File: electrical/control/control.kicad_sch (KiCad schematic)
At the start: 45 parts, among them J1 USB4105-GF-A, J3 SWD, J4 QWIIC, J5 TC2030-NL, J6 UART, SW1 SYS, U1 RP2040, U2 ABPMRRV001PD2A3, U4 W25Q16JVSSIQ, U5 LP5907MFX-3.3, Y1 ABM8-272-T3

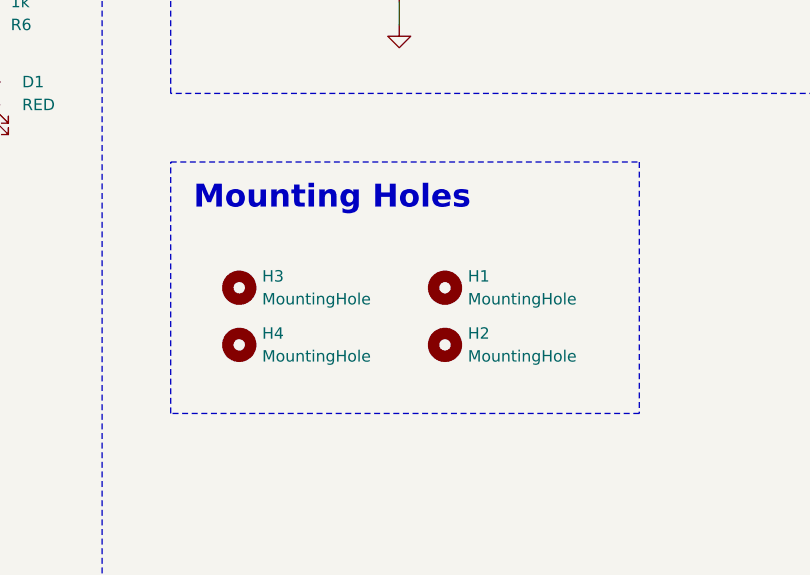
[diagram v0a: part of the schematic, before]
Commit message: Reduce number of mounting holes
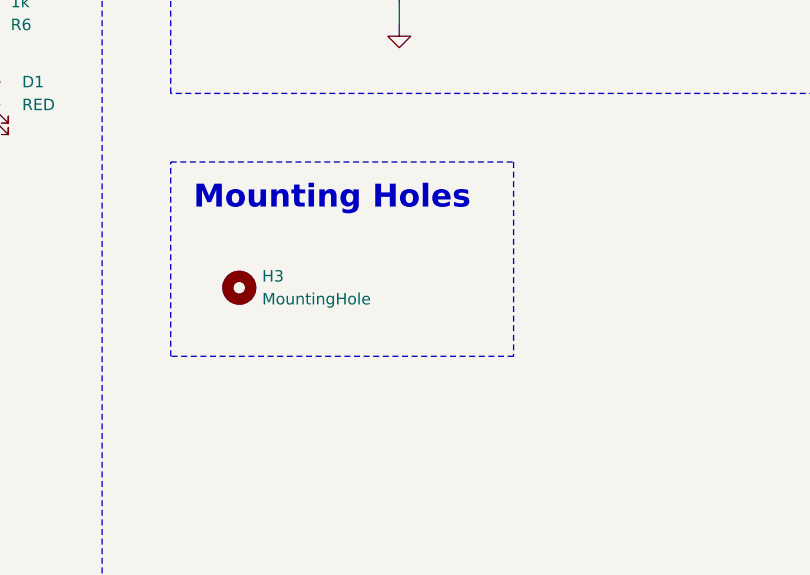
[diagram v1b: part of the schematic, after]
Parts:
- removed H1, H2, H4: MountingHole, MountingHole:MountingHole_3.2mm_M3, symbol Mechanical:MountingHole
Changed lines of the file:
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@@
 	(rectangle
 		(start 300.99 158.75)
-		(end 353.06 186.69)
+		(end 339.09 180.34)
 		(stroke
 			(width 0)
@@
 	)
 	(symbol
-		(lib_id "Mechanical:MountingHole")
-		(at 331.47 172.72 0)
-		(unit 1)
-		(exclude_from_sim no)
-		(in_bom no)
-		(on_board yes)
-		(dnp no)
-		(fields_autoplaced yes)
-		(property "Reference" "H1"
-			(at 334.01 171.4499 0)
-			(effects
-				(font
-					(size 1.27 1.27)
-				)
-				(justify left)
-			)
-		)
-		(property "Value" "MountingHole"
-			(at 334.01 173.9899 0)
-			(effects
-				(font
-					(size 1.27 1.27)
-				)
-				(justify left)
-			)
-		)
-		(property "Footprint" "MountingHole:MountingHole_3.2mm_M3"
-			(at 331.47 172.72 0)
-			(effects
-				(font
-					(size 1.27 1.27)
-				)
-				(hide yes)
-			)
-		)
-		(property "Datasheet" "~"
-			(at 331.47 172.72 0)
-			(effects
-				(font
-					(size 1.27 1.27)
-				)
-				(hide yes)
-			)
-		)
-		(property "Description" "Mounting Hole without connection"
-			(at 331.47 172.72 0)
-			(effects
-				(font
-					(size 1.27 1.27)
-				)
-				(hide yes)
-			)
-		)
-		(instances
-			(project "control"
-				(path "/da26d94e-7a50-4b99-9678-5aaaf6987a15"
-					(reference "H1")
-					(unit 1)
-				)
-			)
-		)
-	)
-	(symbol
 		(lib_id "Device:R_US")
 		(at 105.41 83.82 0)
@@
 	)
 	(symbol
-		(lib_id "Mechanical:MountingHole")
-		(at 308.61 179.07 0)
-		(unit 1)
-		(exclude_from_sim no)
-		(in_bom no)
-		(on_board yes)
-		(dnp no)
-		(fields_autoplaced yes)
-		(property "Reference" "H4"
-			(at 311.15 177.7999 0)
-			(effects
-				(font
-					(size 1.27 1.27)
-				)
-				(justify left)
-			)
-		)
-		(property "Value" "MountingHole"
-			(at 311.15 180.3399 0)
-			(effects
-				(font
-					(size 1.27 1.27)
-				)
-				(justify left)
-			)
-		)
-		(property "Footprint" "MountingHole:MountingHole_3.2mm_M3"
-			(at 308.61 179.07 0)
-			(effects
-				(font
-					(size 1.27 1.27)
-				)
-				(hide yes)
-			)
-		)
-		(property "Datasheet" "~"
-			(at 308.61 179.07 0)
-			(effects
-				(font
-					(size 1.27 1.27)
-				)
-				(hide yes)
-			)
-		)
-		(property "Description" "Mounting Hole without connection"
-			(at 308.61 179.07 0)
-			(effects
-				(font
-					(size 1.27 1.27)
-				)
-				(hide yes)
-			)
-		)
-		(instances
-			(project "control"
-				(path "/da26d94e-7a50-4b99-9678-5aaaf6987a15"
-					(reference "H4")
-					(unit 1)
-				)
-			)
-		)
-	)
-	(symbol
 		(lib_id "Device:R_US")
 		(at 184.15 205.74 0)
@@
 					(unit 1)
 				)
-			)
-		)
-	)
-	(symbol
-		(lib_id "Mechanical:MountingHole")
-		(at 331.47 179.07 0)
-		(unit 1)
-		(exclude_from_sim no)
-		(in_bom no)
-		(on_board yes)
-		(dnp no)
-		(fields_autoplaced yes)
-		(property "Reference" "H2"
-			(at 334.01 177.7999 0)
-			(effects
-				(font
-					(size 1.27 1.27)
-				)
-				(justify left)
-			)
-		)
-		(property "Value" "MountingHole"
-			(at 334.01 180.3399 0)
-			(effects
-				(font
-					(size 1.27 1.27)
-				)
-				(justify left)
-			)
-		)
-		(property "Footprint" "MountingHole:MountingHole_3.2mm_M3"
-			(at 331.47 179.07 0)
-			(effects
-				(font
-					(size 1.27 1.27)
-				)
-				(hide yes)
-			)
-		)
-		(property "Datasheet" "~"
-			(at 331.47 179.07 0)
-			(effects
-				(font
-					(size 1.27 1.27)
-				)
-				(hide yes)
-			)
-		)
-		(property "Description" "Mounting Hole without connection"
-			(at 331.47 179.07 0)
-			(effects
-				(font
-					(size 1.27 1.27)
-				)
-				(hide yes)
-			)
-		)
-		(instances
-			(project "control"
-				(path "/da26d94e-7a50-4b99-9678-5aaaf6987a15"
-					(reference "H2")
-					(unit 1)
-				)
